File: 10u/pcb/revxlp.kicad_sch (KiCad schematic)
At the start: 189 parts, among them Q1 AO3416 N-channel MOSFET, SW1 SW_SPDT, SW2 SW_Push, U1 74HC595, U2 SeeeduinoXIAO_BLE

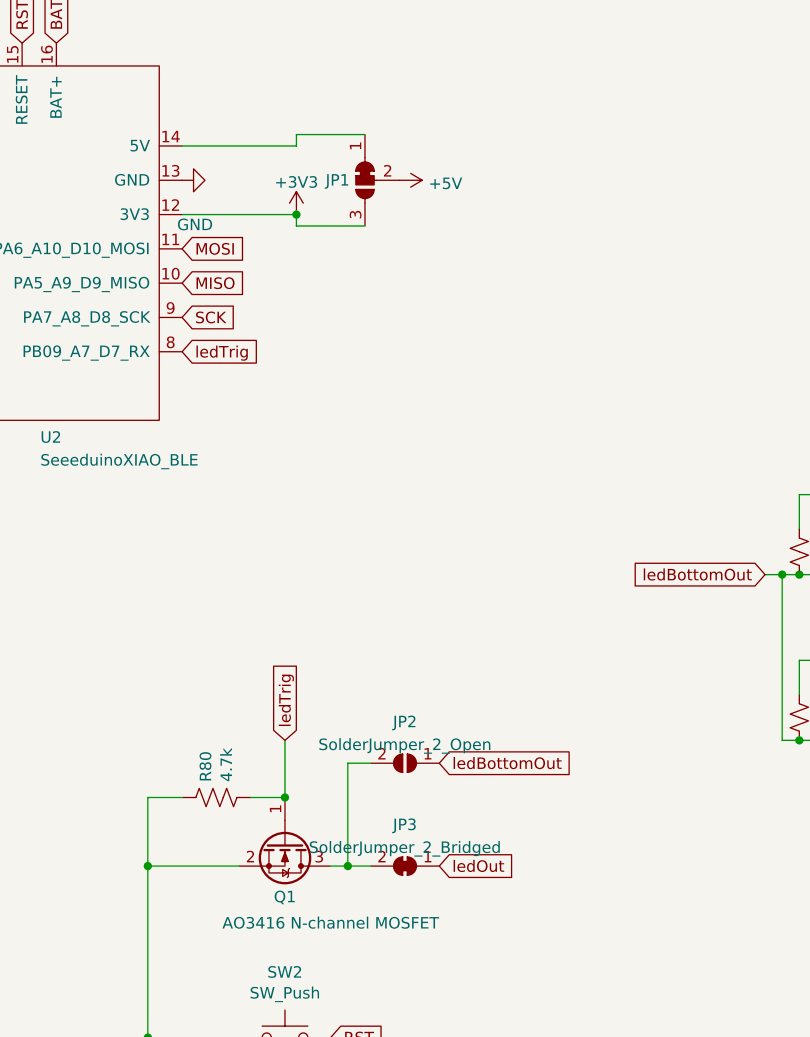
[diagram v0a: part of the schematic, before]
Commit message: Silk cleanup.
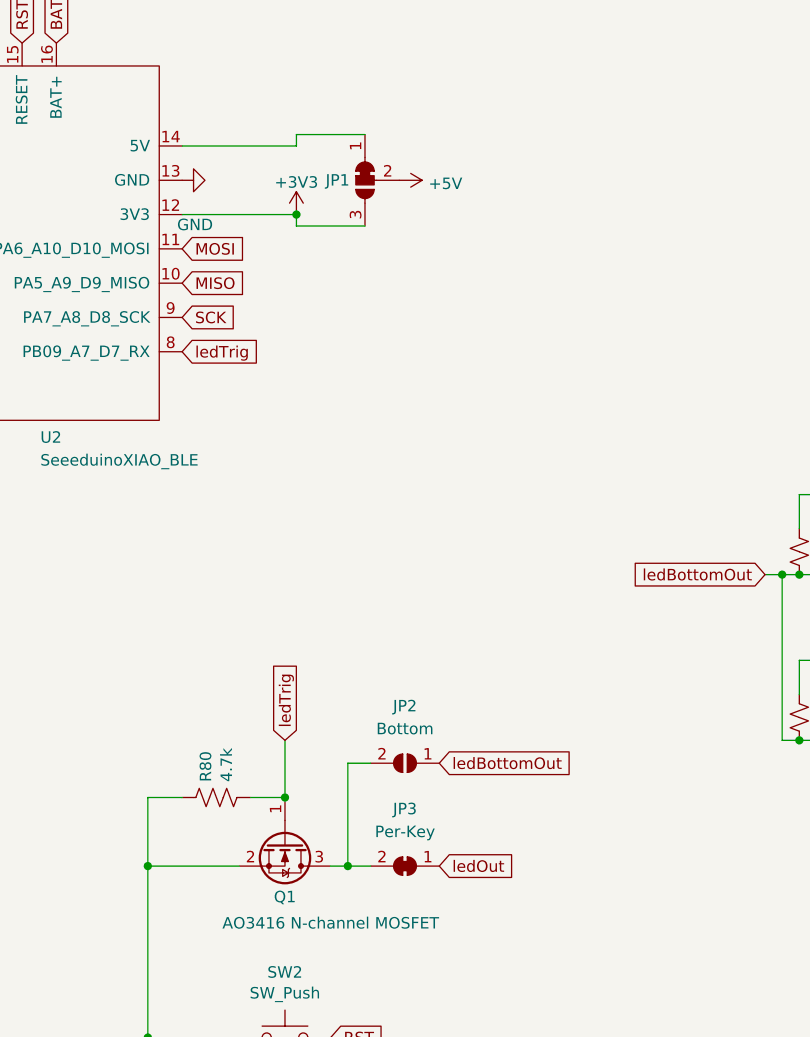
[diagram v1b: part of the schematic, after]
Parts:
- JP2: value SolderJumper_2_Open -> Bottom
- JP3: value SolderJumper_2_Bridged -> Per-Key
